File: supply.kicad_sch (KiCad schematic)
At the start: 43 parts, among them U1 AP62301_TSOT, U2 AP62301_TSOT, U3 NCP163ASN330T1G, U4 REF3012AIDBZT, U5 TLV73312PDBVT

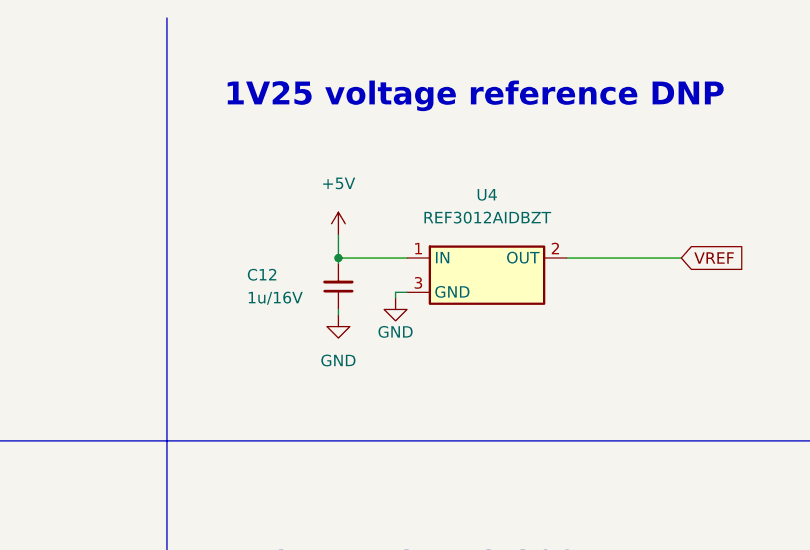
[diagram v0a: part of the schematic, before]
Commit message: [#53377] Mark 1V25 reference as DNP
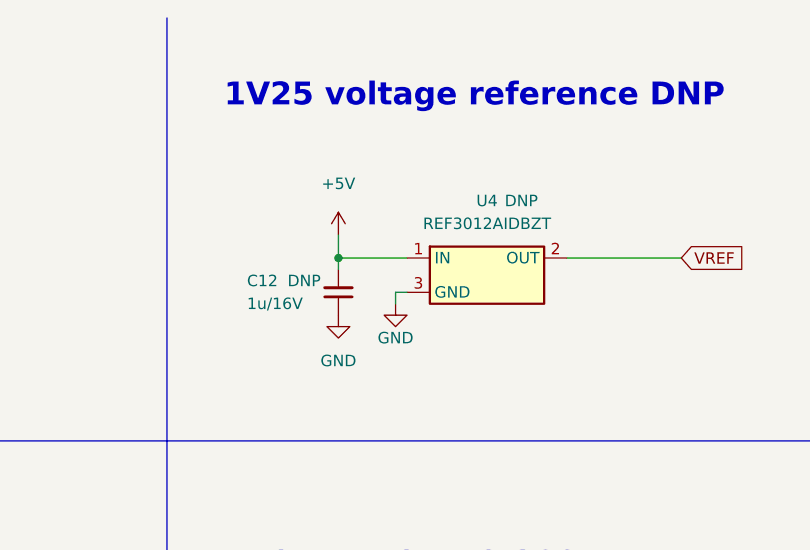
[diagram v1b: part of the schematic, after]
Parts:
- C12, U4: DNP (none) -> DNP
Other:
- moved on the sheet: C12
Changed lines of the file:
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@@
     (stroke (width 0) (type default) (color 0 0 0 0))
   )
-  (wire (pts (xy 179.07 45.085) (xy 179.07 45.72))
-    (stroke (width 0) (type default) (color 0 0 0 0))
-  )
   (wire (pts (xy 46.99 104.14) (xy 46.99 102.87))
     (stroke (width 0) (type default) (color 0 0 0 0))
@@
     (stroke (width 0) (type default) (color 0 0 0 0))
   )
-  (wire (pts (xy 179.07 39.37) (xy 179.07 40.005))
+  (wire (pts (xy 179.07 39.37) (xy 179.07 40.64))
     (stroke (width 0) (type default) (color 0 0 0 0))
   )
@@
     (stroke (width 0) (type default) (color 0 0 0 0))
   )
-  (wire (pts (xy 185.42 43.18) (xy 185.42 43.815))
+  (wire (pts (xy 185.42 43.18) (xy 185.42 44.45))
     (stroke (width 0) (type default) (color 0 0 0 0))
   )
@@
   )
   (symbol (lib_id "antmicroPMICVoltageRegulatorsLinear:TLV73312PDBVT") (at 187.96 95.25 0) (unit 1)
-    (in_bom yes) (on_board yes) (fields_autoplaced)
+    (in_bom yes) (on_board yes)
     (property "Reference" "U5" (id 0) (at 198.12 87.63 0)
       (effects (font (size 1.27 1.27) (thickness 0.15)))
@@
   )
   (symbol (lib_id "antmicroPMICPowerDistributionSwitchesLoadDrivers:REF3012AIDBZT") (at 186.69 39.37 0) (unit 1)
-    (in_bom yes) (on_board yes) (fields_autoplaced)
-    (property "Reference" "U4" (id 0) (at 195.58 32.385 0)
+    (in_bom yes) (on_board yes)
+    (property "Reference" "U4" (id 0) (at 195.58 33.02 0)
       (effects (font (size 1.27 1.27) (thickness 0.15)))
     )
-    (property "Value" "REF3012AIDBZT" (id 1) (at 195.58 34.925 0)
+    (property "Value" "REF3012AIDBZT" (id 1) (at 195.58 35.56 0)
       (effects (font (size 1.27 1.27) (thickness 0.15)))
     )
@@
       (effects (font (size 1.27 1.27) (thickness 0.15)) (justify left bottom) hide)
     )
+    (property "DNP" "DNP" (id 8) (at 199.39 33.02 0))
     (pin "1")
     (pin "2")
@@
     (pin "2")
   )
-  (symbol (lib_id "antmicroCapacitors0402:C_1u_16V_0402") (at 179.07 45.085 90) (unit 1)
+  (symbol (lib_id "antmicroCapacitors0402:C_1u_16V_0402") (at 179.07 45.72 90) (unit 1)
     (in_bom yes) (on_board yes)
-    (property "Reference" "C12" (id 0) (at 168.91 41.275 90)
+    (property "Reference" "C12" (id 0) (at 168.91 41.91 90)
       (effects (font (size 1.27 1.27) (thickness 0.15)) (justify right))
     )
-    (property "Value" "C_1u_16V_0402" (id 1) (at 189.23 24.765 0)
+    (property "Value" "C_1u_16V_0402" (id 1) (at 189.23 25.4 0)
       (effects (font (size 1.27 1.27) (thickness 0.15)) (justify left bottom) hide)
     )
-    (property "Footprint" "antmicro-footprints:C_0402_1005Metric" (id 2) (at 191.77 24.765 0)
+    (property "Footprint" "antmicro-footprints:C_0402_1005Metric" (id 2) (at 191.77 25.4 0)
       (effects (font (size 1.27 1.27) (thickness 0.15)) (justify left bottom) hide)
     )
-    (property "Datasheet" "https://www.kemet.com/en/us/capacitors/product/C0402C105M4PACTU.html" (id 3) (at 194.31 24.765 0)
+    (property "Datasheet" "https://www.kemet.com/en/us/capacitors/product/C0402C105M4PACTU.html" (id 3) (at 194.31 25.4 0)
       (effects (font (size 1.27 1.27) (thickness 0.15)) (justify left bottom) hide)
     )
-    (property "MPN" "C0402C105M4PACTU" (id 4) (at 196.85 24.765 0)
+    (property "MPN" "C0402C105M4PACTU" (id 4) (at 196.85 25.4 0)
       (effects (font (size 1.27 1.27) (thickness 0.15)) (justify left bottom) hide)
     )
-    (property "Manufacturer" "KEMET" (id 5) (at 199.39 24.765 0)
+    (property "Manufacturer" "KEMET" (id 5) (at 199.39 25.4 0)
       (effects (font (size 1.27 1.27) (thickness 0.15)) (justify left bottom) hide)
     )
-    (property "License" "Apache-2.0" (id 6) (at 201.93 24.765 0)
+    (property "License" "Apache-2.0" (id 6) (at 201.93 25.4 0)
       (effects (font (size 1.27 1.27) (thickness 0.15)) (justify left bottom) hide)
     )
-    (property "Author" "Antmicro" (id 7) (at 204.47 24.765 0)
+    (property "Author" "Antmicro" (id 7) (at 204.47 25.4 0)
       (effects (font (size 1.27 1.27) (thickness 0.15)) (justify left bottom) hide)
     )
-    (property "Val" "1u/16V" (id 8) (at 168.91 43.815 90)
+    (property "Val" "1u/16V" (id 8) (at 168.91 44.45 90)
       (effects (font (size 1.27 1.27) (thickness 0.15)) (justify right))
     )
-    (property "Voltage" "" (id 9) (at 207.01 24.765 0)
+    (property "Voltage" "" (id 9) (at 207.01 25.4 0)
       (effects (font (size 1.27 1.27)) (justify left bottom) hide)
     )
-    (property "Dielectric" "" (id 10) (at 209.55 24.765 0)
+    (property "Dielectric" "" (id 10) (at 209.55 25.4 0)
       (effects (font (size 1.27 1.27)) (justify left bottom) hide)
     )
+    (property "DNP" "DNP" (id 11) (at 175.26 41.91 90))
     (pin "1")
     (pin "2")
@@
     (pin "6")
   )
-  (symbol (lib_id "antmicropower:GND") (at 185.42 43.815 0) (mirror y) (unit 1)
+  (symbol (lib_id "antmicropower:GND") (at 185.42 44.45 0) (mirror y) (unit 1)
     (in_bom yes) (on_board yes)
-    (property "Reference" "#PWR0108" (id 0) (at 176.53 46.355 0)
+    (property "Reference" "#PWR0108" (id 0) (at 176.53 46.99 0)
       (effects (font (size 1.27 1.27) (thickness 0.15)) (justify left bottom) hide)
     )
-    (property "Value" "GND" (id 1) (at 185.42 47.625 0)
+    (property "Value" "GND" (id 1) (at 185.42 48.26 0)
       (effects (font (size 1.27 1.27) (thickness 0.15)))
     )
-    (property "Footprint" "" (id 2) (at 176.53 51.435 0)
+    (property "Footprint" "" (id 2) (at 176.53 52.07 0)
       (effects (font (size 1.27 1.27) (thickness 0.15)) (justify left bottom) hide)
     )
-    (property "Datasheet" "" (id 3) (at 176.53 56.515 0)
+    (property "Datasheet" "" (id 3) (at 176.53 57.15 0)
       (effects (font (size 1.27 1.27) (thickness 0.15)) (justify left bottom) hide)
     )
-    (property "Author" "Antmicro" (id 4) (at 176.53 51.435 0)
+    (property "Author" "Antmicro" (id 4) (at 176.53 52.07 0)
       (effects (font (size 1.27 1.27) (thickness 0.15)) (justify left bottom) hide)
     )
-    (property "License" "Apache-2.0" (id 5) (at 176.53 53.975 0)
+    (property "License" "Apache-2.0" (id 5) (at 176.53 54.61 0)
       (effects (font (size 1.27 1.27) (thickness 0.15)) (justify left bottom) hide)
     )
